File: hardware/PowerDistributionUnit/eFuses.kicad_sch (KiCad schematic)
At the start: 13 parts, among them U3 TCA9544A, U36 MCP23S17-E/SS

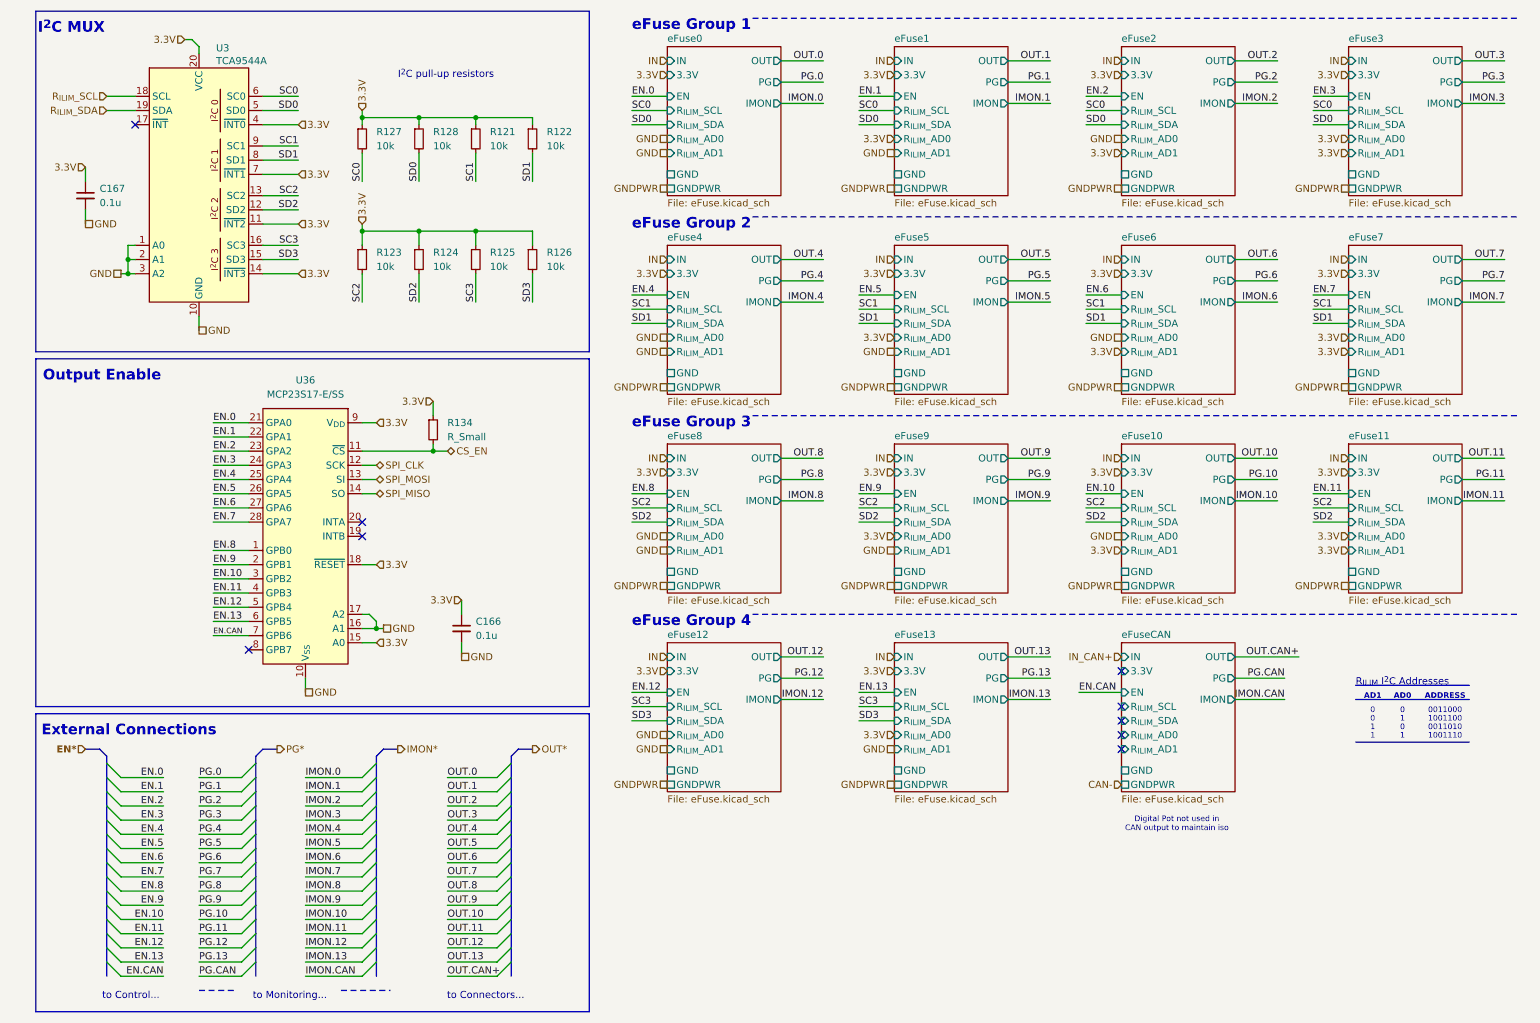
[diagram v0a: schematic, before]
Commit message: schematic updated
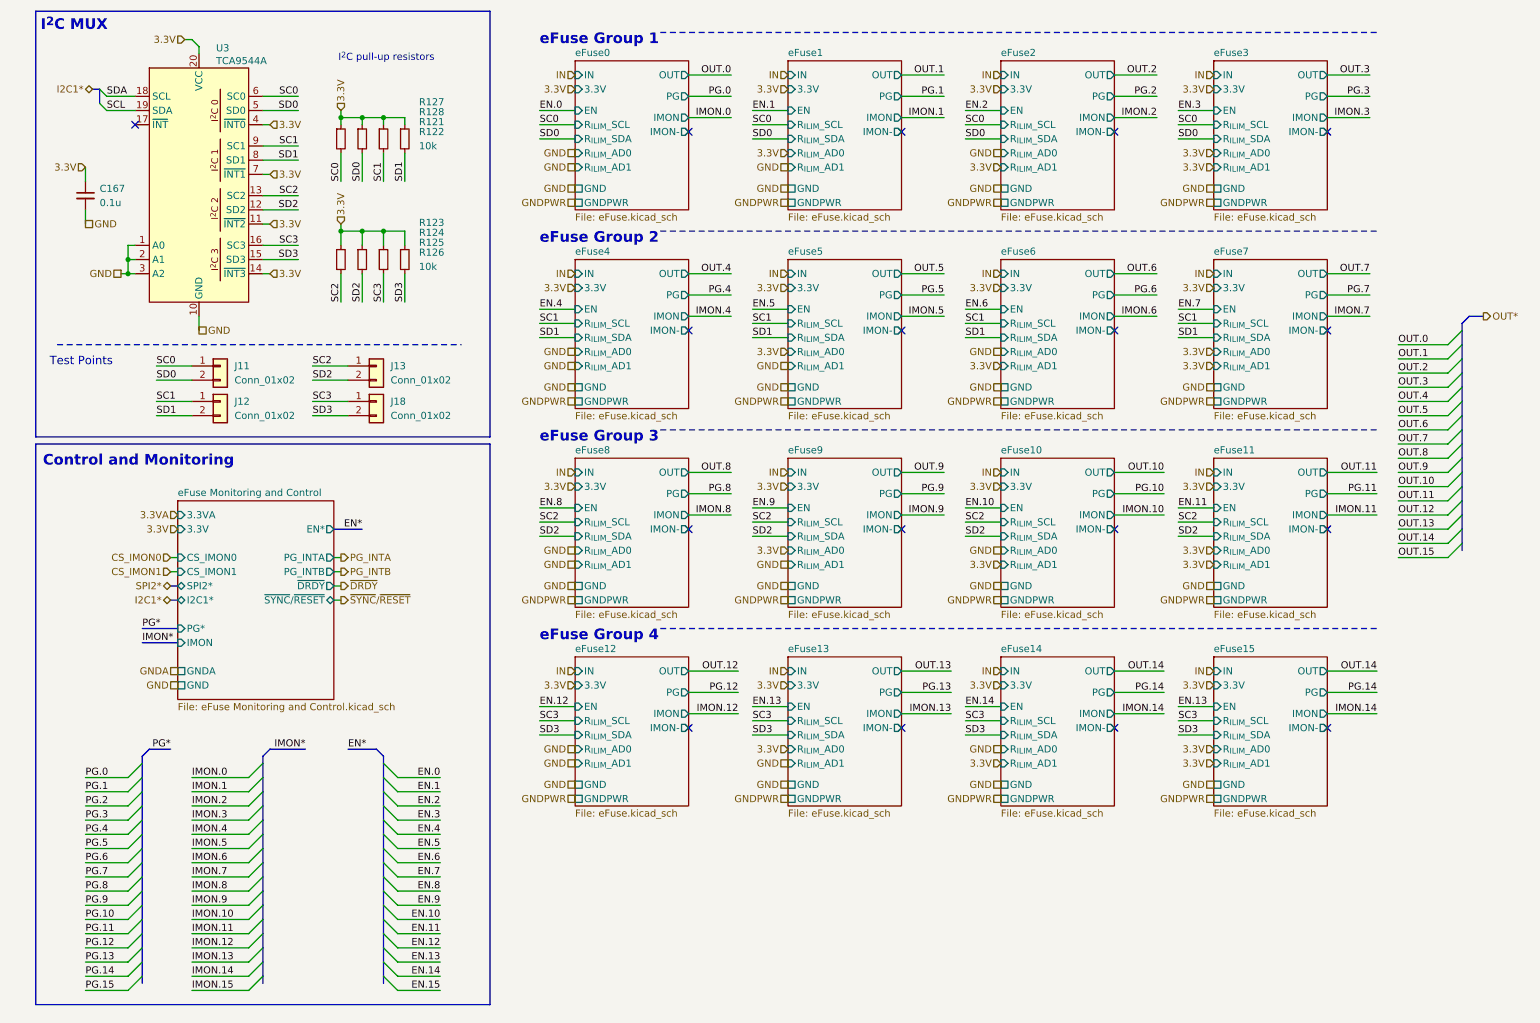
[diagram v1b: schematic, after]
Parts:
- removed C166: 0.1u, symbol Device:C_Small
- removed R134: R_Small, symbol Device:R_Small
- removed U36: MCP23S17-E/SS, Package_SO:SSOP-28_5.3x10.2mm_P0.65mm, symbol PowerDistributionUnitLib:MCP23S17-E/SS
- added J11, J12, J13, J18: Conn_01x02, Connector_PinHeader_2.54mm:PinHeader_1x02_P2.54mm_Vertical, symbol Connector_Generic:Conn_01x02
- C167: footprint (none) -> Capacitor_SMD:C_0603_1608Metric
- R121, R122, R123, R124, R125, R126, R127, R128: footprint (none) -> Resistor_SMD:R_0603_1608Metric
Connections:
- net SC0: now also J11.1 (Pin_1)
- net SC1: now also J12.1 (Pin_1)
- net SC2: now also J13.1 (Pin_1)
- net SC3: now also J18.1 (Pin_1)
- net SD0: now also J11.2 (Pin_2)
- net SD1: now also J12.2 (Pin_2)
- net SD2: now also J13.2 (Pin_2)
- net SD3: now also J18.2 (Pin_2)
- net R_{ILIM}_SCL renamed SDA
- net R_{ILIM}_SDA renamed SCL
- no-connect marks 9 -> 17
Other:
- removed sheet eFuseCAN
- added sheet eFuse Monitoring and Control (eFuse Monitoring and Control.kicad_sch)
- added sheet eFuse14 (eFuse.kicad_sch)
- added sheet eFuse15 (eFuse.kicad_sch)
- sheet eFuse0 ports: added IMON-; removed none
- sheet eFuse1 ports: added IMON-; removed none
- sheet eFuse10 ports: added IMON-; removed none
- sheet eFuse11 ports: added IMON-; removed none
- sheet eFuse12 ports: added IMON-; removed none
- sheet eFuse13 ports: added IMON-; removed none
- sheet eFuse2 ports: added IMON-; removed none
- sheet eFuse3 ports: added IMON-; removed none
- sheet eFuse4 ports: added IMON-; removed none
- sheet eFuse5 ports: added IMON-; removed none
- sheet eFuse6 ports: added IMON-; removed none
- sheet eFuse7 ports: added IMON-; removed none
- sheet eFuse8 ports: added IMON-; removed none
- sheet eFuse9 ports: added IMON-; removed none
- note added: "Control and Monitoring"
- note added: "Test Points"
- note removed: "0"
- note removed: "0011000"
- note removed: "0011010"
- note removed: "1"
- note removed: "1001100"
- note removed: "1001110"
- note removed: "AD0"
- note removed: "AD1"
- note removed: "ADDRESS"
- note removed: "Digital Pot not used in CAN output to maintain iso"
- note removed: "External Connections"
- note removed: "Output Enable"
- note removed: "R_{ILIM} I^{2}C Addresses"
- note removed: "to Connectors..."
- note removed: "to Control..."
- note removed: "to Monitoring..."
- company: (none) -> Longhorn Racing
- title: (none) -> eFuses
- moved on the sheet: R121, R122, R123, R124, R125, R126, R127, R128
